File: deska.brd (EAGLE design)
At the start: 100 x 80 mm, 17 parts, among them Q1 BC547, Q2 BC547

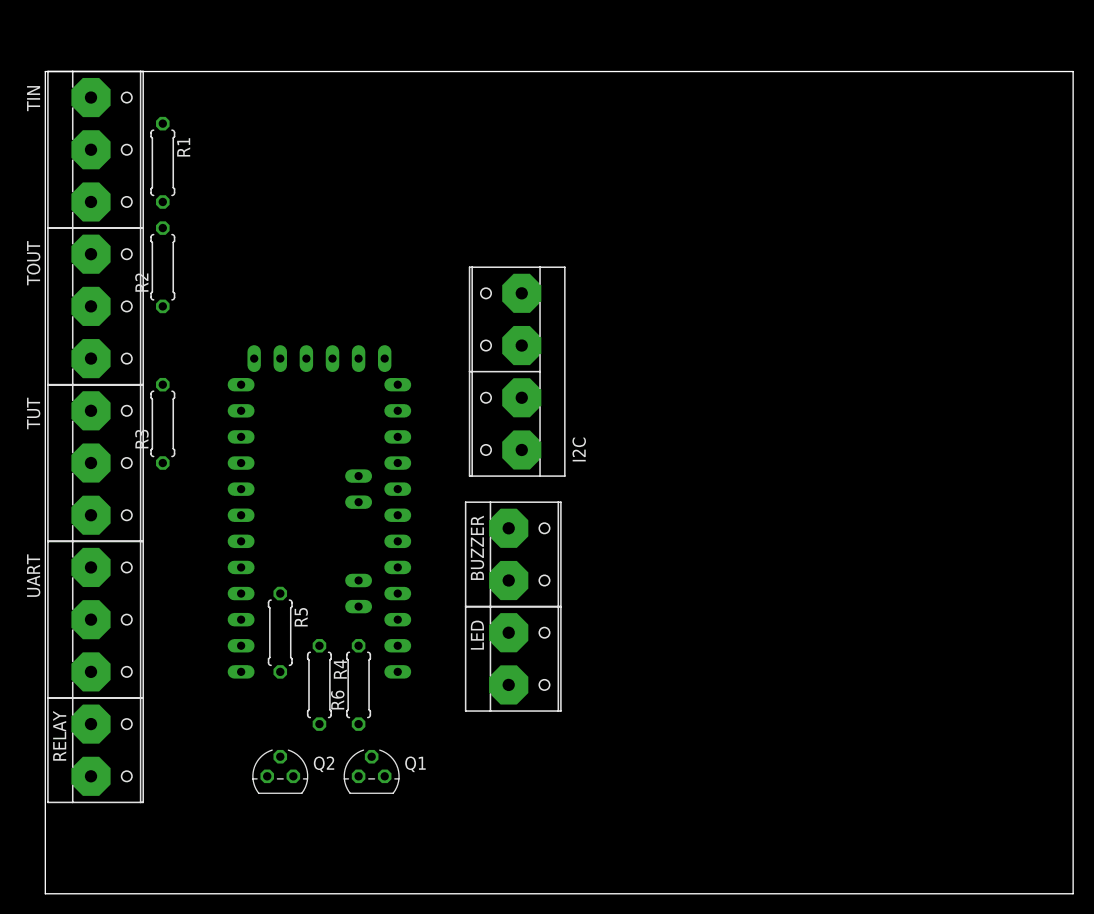
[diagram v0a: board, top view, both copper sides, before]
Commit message: zmeny
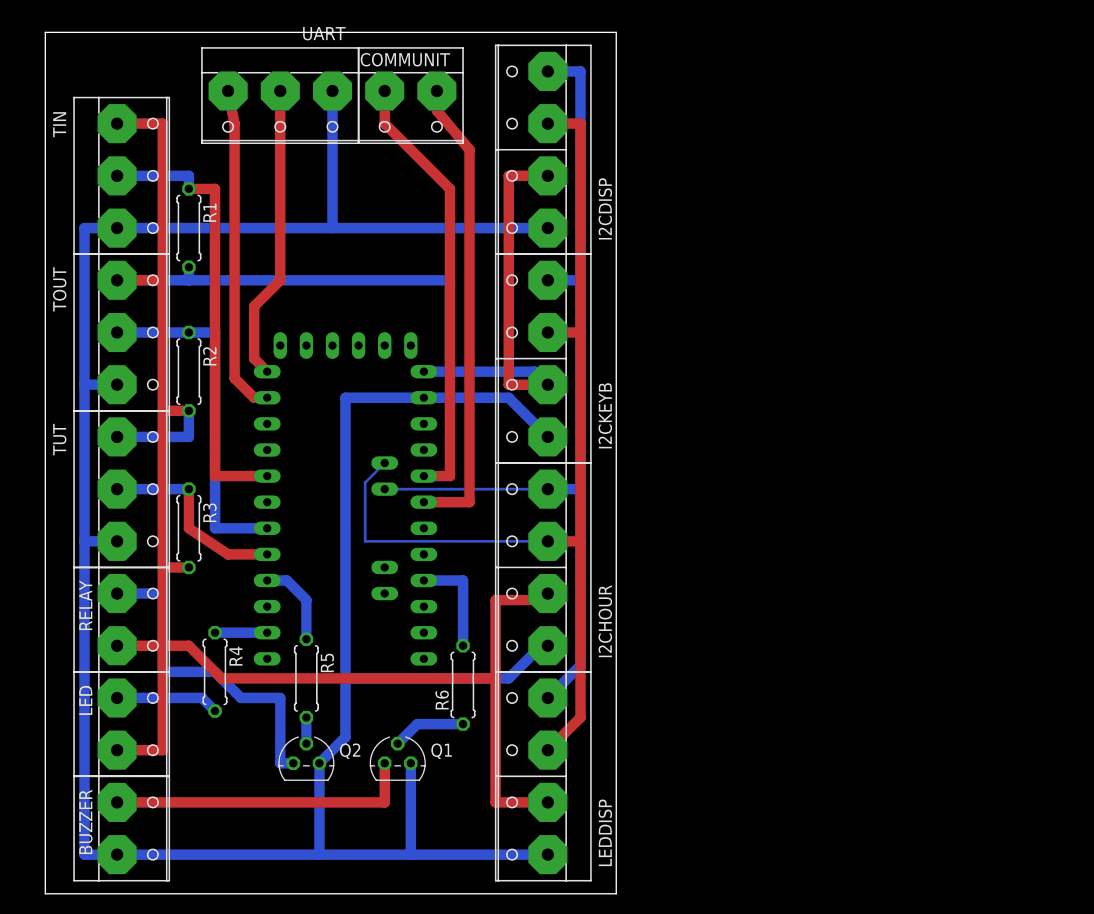
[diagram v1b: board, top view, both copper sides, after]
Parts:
- removed I2C: (no value), con-wago-508:W237-4P
- added COMMUNIT: (no value), con-wago-508:W237-132
- added I2CDISP, I2CHOUR, I2CKEYB, LEDDISP: (no value), con-wago-508:W237-4P
- moved UART 53.8 mm to (22.9, 77.5), turned to 180 degrees
- moved BUZZER 46.5 mm to (7.62, 6.35)
- moved LED 38.6 mm to (7.62, 16.5)
- moved RELAY 13.0 mm to (7.62, 26.7)
- moved R2 10.5 mm to (14.0, 50.8), turned to 270 degrees
- moved R3 10.5 mm to (14.0, 35.6), turned to 270 degrees
- moved R4 10.2 mm to (16.5, 21.6)
- moved R6 10.2 mm to (40.6, 20.3)
- moved R1 6.84 mm to (14.0, 64.8)
- moved R5 5.12 mm to (25.4, 21.0)
- moved TIN 3.59 mm to (7.62, 69.8)
- moved TOUT 3.59 mm to (7.62, 54.6)
- moved TUT 3.59 mm to (7.62, 39.4)
- moved U$1 2.84 mm to (30.5, 38.1)
- moved Q1 2.84 mm to (34.3, 12.7)
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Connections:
- new net N$17: COMMUNIT.2, U$1.A0
- new net N$8: COMMUNIT.1, U$1.A1
- net +5V: now also I2CDISP.2, I2CHOUR.2, I2CKEYB.2, LEDDISP.2; no longer I2C.2
- net GND: now also I2CDISP.1, I2CHOUR.1, I2CKEYB.1, LEDDISP.1, TIN.3; no longer I2C.1, TIN.2
- net N$1: now also TIN.2; no longer TIN.3
- net N$11: now also I2CDISP.4, I2CHOUR.4, I2CKEYB.4, LEDDISP.4; no longer I2C.4
- net N$12: now also I2CDISP.3, I2CHOUR.3, I2CKEYB.3, LEDDISP.3; no longer I2C.3
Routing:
- net GND: track 0.00 -> 268.1 mm
- net +5V: track 0.00 -> 240.2 mm
- net N$12: track 0.00 -> 98.0 mm
- net N$11: track 0.00 -> 87.7 mm
- net N$8: track 0.00 -> 45.6 mm
- net N$1: track 0.00 -> 43.8 mm
- net N$17: track 0.00 -> 42.6 mm
- net N$2: track 0.00 -> 33.7 mm
- net N$14: track 0.00 -> 32.2 mm
- net N$10: track 0.00 -> 32.0 mm
- net N$15: track 0.00 -> 29.8 mm
- net N$9: track 0.00 -> 28.9 mm
- net N$3: track 0.00 -> 19.2 mm
- net N$16: track 0.00 -> 10.2 mm
- net N$6: track 0.00 -> 10.1 mm
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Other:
- board size 100 x 80 mm -> 55.5 x 83.8 mm
